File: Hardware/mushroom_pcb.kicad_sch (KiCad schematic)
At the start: 52 parts, among them J1 Conn_01x04, J2 Conn_01x07_Pin, J3 Screw_Terminal_01x03, J4 Screw_Terminal_01x02, J5 Screw_Terminal_01x02, J6 Screw_Terminal_01x03, J7 Conn_01x03_Pin, J8 Conn_01x04_Pin, J9 Barrel_Jack, Q3 AO3400A, Q4 AO3400A, SW1 SW_Push, SW2 SW_Push, SW3 RotaryEncoder_Switch, U1 ESP32-WROOM-32E, U2 LM2596S-5, U3 ME6211C33M5

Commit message: Nueva version más compacta y con elementos handsoldering (falta rutear y cambiar algunas huellas)
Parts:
- R1: footprint Resistor_SMD:R_0508_1220Metric -> Resistor_SMD:R_0805_2012Metric_Pad1.20x1.40mm_HandSolder
- R10, R11, R12, R13, R14, R15, R5, R6, R7, R8, R9: footprint Resistor_SMD:R_0805_2012Metric -> Resistor_SMD:R_0805_2012Metric_Pad1.20x1.40mm_HandSolder
- R2, R3, R4: footprint Resistor_SMD:R_0603_1608Metric -> Resistor_SMD:R_0805_2012Metric_Pad1.20x1.40mm_HandSolder
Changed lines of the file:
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@@
 			)
 		)
-		(property "Footprint" "Resistor_SMD:R_0603_1608Metric"
+		(property "Footprint" "Resistor_SMD:R_0805_2012Metric_Pad1.20x1.40mm_HandSolder"
 			(at 103.632 115.57 90)
 			(hide yes)
@@
 			)
 		)
-		(property "Footprint" "Resistor_SMD:R_0508_1220Metric"
+		(property "Footprint" "Resistor_SMD:R_0805_2012Metric_Pad1.20x1.40mm_HandSolder"
 			(at 66.04 57.912 90)
 			(hide yes)
@@
 			)
 		)
-		(property "Footprint" "Resistor_SMD:R_0603_1608Metric"
+		(property "Footprint" "Resistor_SMD:R_0805_2012Metric_Pad1.20x1.40mm_HandSolder"
 			(at 111.252 115.57 90)
 			(hide yes)
@@
 			)
 		)
-		(property "Footprint" "Resistor_SMD:R_0805_2012Metric"
+		(property "Footprint" "Resistor_SMD:R_0805_2012Metric_Pad1.20x1.40mm_HandSolder"
 			(at 21.082 171.45 90)
 			(hide yes)
@@
 			)
 		)
-		(property "Footprint" "Resistor_SMD:R_0805_2012Metric"
+		(property "Footprint" "Resistor_SMD:R_0805_2012Metric_Pad1.20x1.40mm_HandSolder"
 			(at 167.64 81.788 90)
 			(hide yes)
@@
 			)
 		)
-		(property "Footprint" "Resistor_SMD:R_0805_2012Metric"
+		(property "Footprint" "Resistor_SMD:R_0805_2012Metric_Pad1.20x1.40mm_HandSolder"
 			(at 199.39 145.288 90)
 			(hide yes)
@@
 			)
 		)
-		(property "Footprint" "Resistor_SMD:R_0805_2012Metric"
+		(property "Footprint" "Resistor_SMD:R_0805_2012Metric_Pad1.20x1.40mm_HandSolder"
 			(at 66.802 172.72 90)
 			(hide yes)
@@
 			)
 		)
-		(property "Footprint" "Resistor_SMD:R_0805_2012Metric"
+		(property "Footprint" "Resistor_SMD:R_0805_2012Metric_Pad1.20x1.40mm_HandSolder"
 			(at 201.422 118.11 90)
 			(hide yes)
@@
 			)
 		)
-		(property "Footprint" "Resistor_SMD:R_0805_2012Metric"
+		(property "Footprint" "Resistor_SMD:R_0805_2012Metric_Pad1.20x1.40mm_HandSolder"
 			(at 202.692 151.13 90)
 			(hide yes)
@@
 			)
 		)
-		(property "Footprint" "Resistor_SMD:R_0805_2012Metric"
+		(property "Footprint" "Resistor_SMD:R_0805_2012Metric_Pad1.20x1.40mm_HandSolder"
 			(at 198.12 112.268 90)
 			(hide yes)
@@
 			)
 		)
-		(property "Footprint" "Resistor_SMD:R_0805_2012Metric"
+		(property "Footprint" "Resistor_SMD:R_0805_2012Metric_Pad1.20x1.40mm_HandSolder"
 			(at 50.292 171.45 90)
 			(hide yes)
@@
 			)
 		)
-		(property "Footprint" "Resistor_SMD:R_0805_2012Metric"
+		(property "Footprint" "Resistor_SMD:R_0805_2012Metric_Pad1.20x1.40mm_HandSolder"
 			(at 80.772 172.72 90)
 			(hide yes)
@@
 			)
 		)
-		(property "Footprint" "Resistor_SMD:R_0603_1608Metric"
+		(property "Footprint" "Resistor_SMD:R_0805_2012Metric_Pad1.20x1.40mm_HandSolder"
 			(at 140.462 120.65 90)
 			(hide yes)
@@
 			)
 		)
-		(property "Footprint" "Resistor_SMD:R_0805_2012Metric"
+		(property "Footprint" "Resistor_SMD:R_0805_2012Metric_Pad1.20x1.40mm_HandSolder"
 			(at 237.49 30.988 90)
 			(hide yes)
@@
 			)
 		)
-		(property "Footprint" "Resistor_SMD:R_0805_2012Metric"
+		(property "Footprint" "Resistor_SMD:R_0805_2012Metric_Pad1.20x1.40mm_HandSolder"
 			(at 35.052 171.45 90)
 			(hide yes)

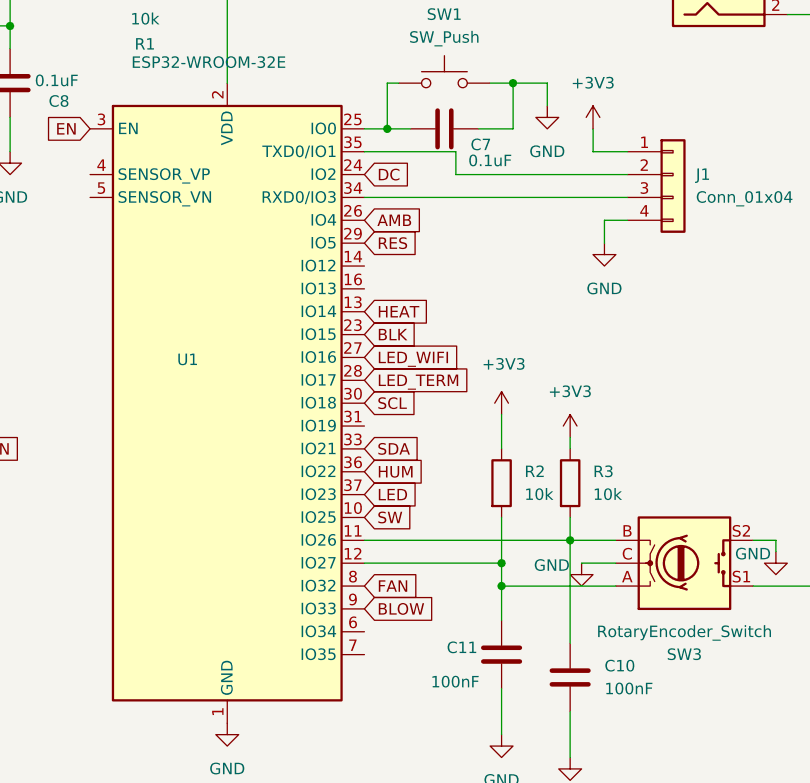
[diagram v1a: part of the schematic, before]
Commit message: Re ruteo placa
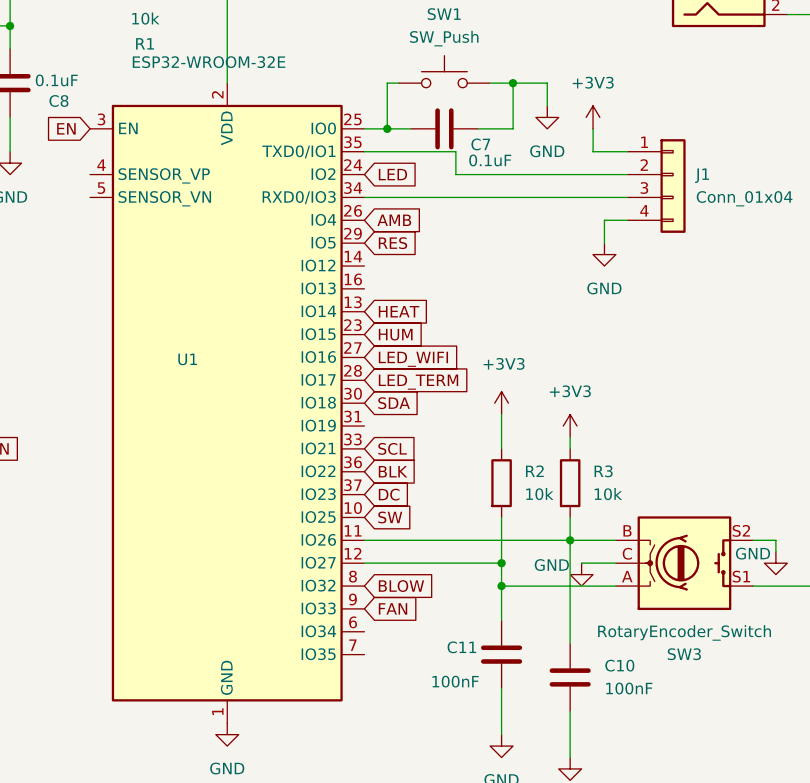
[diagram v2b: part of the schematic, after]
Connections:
- net BLK: now also U1.36 (IO22); no longer U1.23 (IO15)
- net BLOW: now also U1.8 (IO32); no longer U1.9 (IO33)
- net DC: now also U1.37 (IO23); no longer U1.24 (IO2)
- net FAN: now also U1.9 (IO33); no longer U1.8 (IO32)
- net HUM: now also U1.23 (IO15); no longer U1.36 (IO22)
- net LED: now also U1.24 (IO2); no longer U1.37 (IO23)
- net SCL: now also U1.33 (IO21); no longer U1.30 (IO18)
- net SDA: now also U1.30 (IO18); no longer U1.33 (IO21)
